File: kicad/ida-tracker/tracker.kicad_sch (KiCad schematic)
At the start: 1 part, among them J1 EURO_PWR_2x5

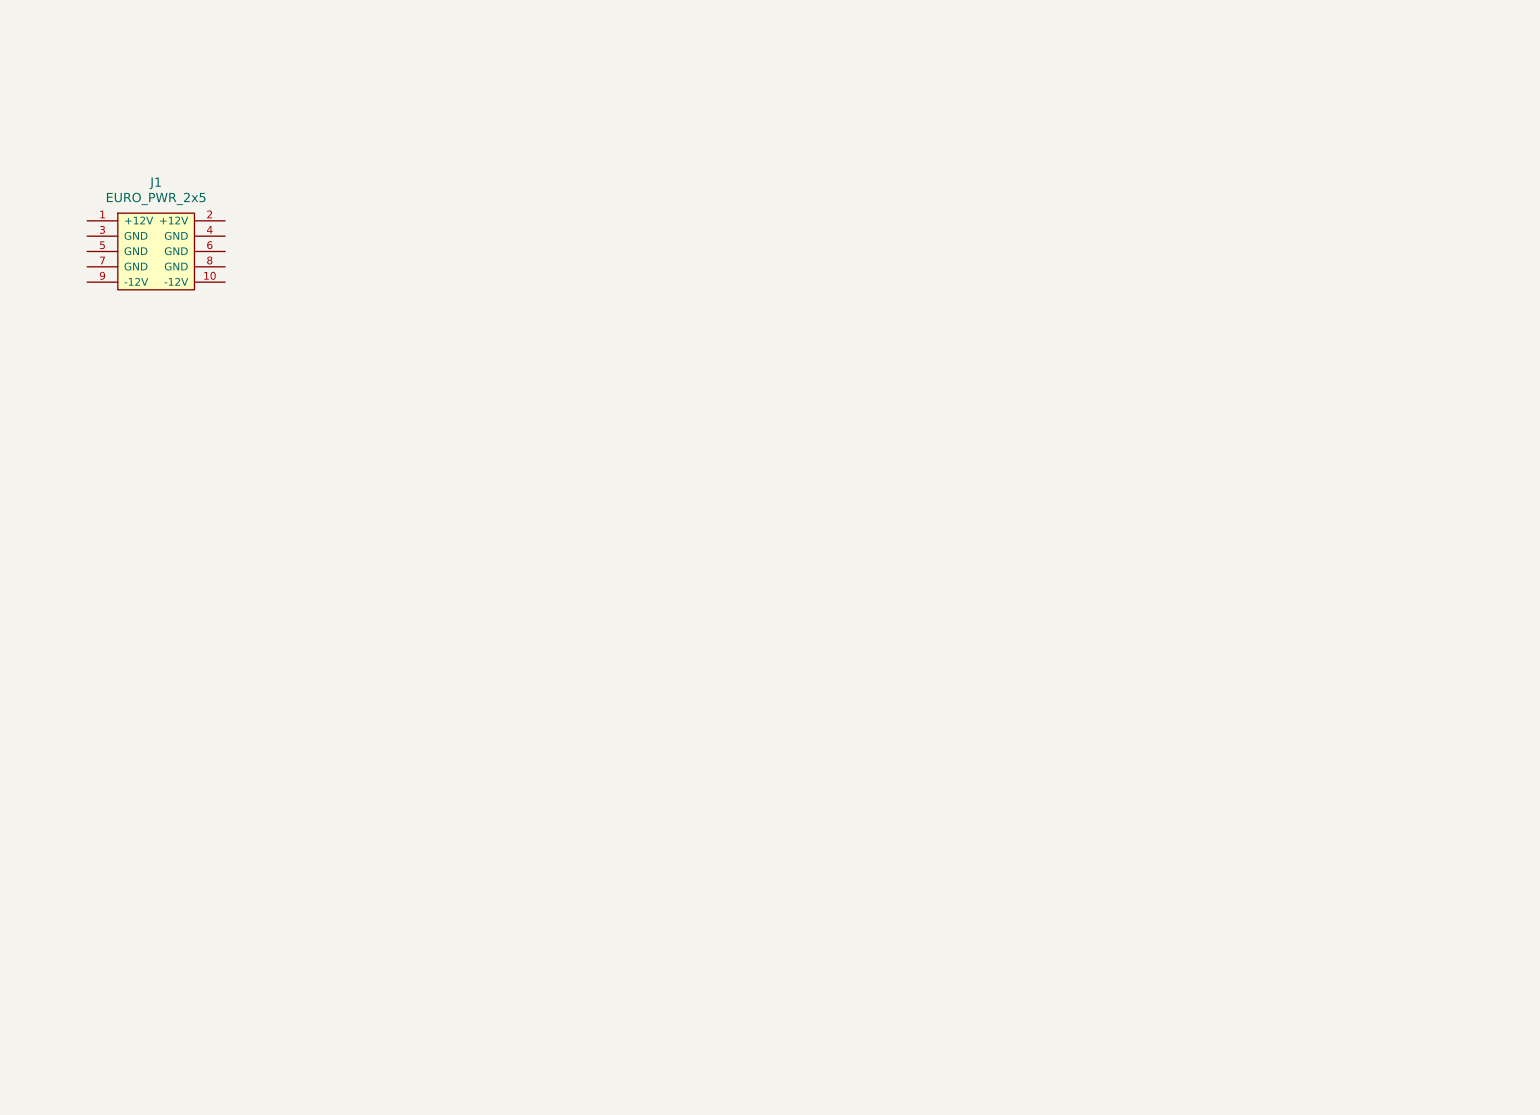
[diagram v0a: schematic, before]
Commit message: stylophone rev1
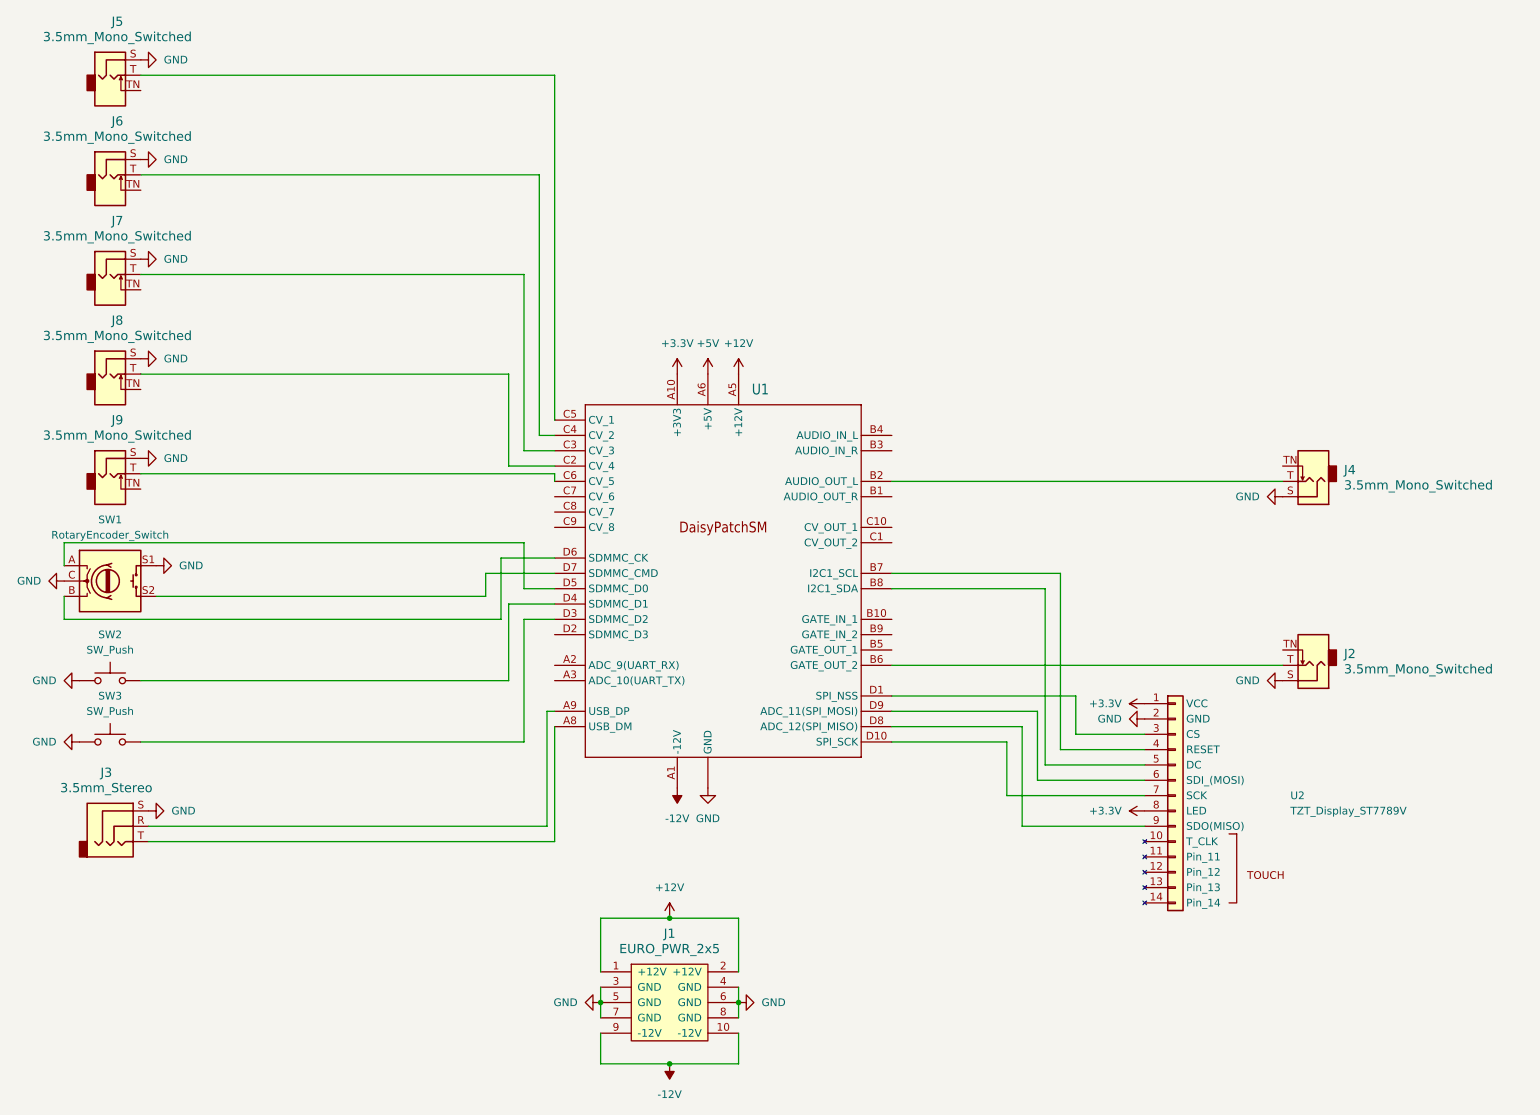
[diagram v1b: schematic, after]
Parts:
- added J2, J4, J5, J6, J7, J8, J9: 3.5mm_Mono_Switched, Connector_Audio:Jack_3.5mm_QingPu_WQP-PJ398SM_Vertical_CircularHoles, symbol KitsBlips:3.5mm_Mono_Switched
- added J3: 3.5mm_Stereo, KitsBlips:Stereo_Thonk_PJ366ST, symbol KitsBlips:3.5mm_Stereo
- added SW1: RotaryEncoder_Switch, Rotary_Encoder:RotaryEncoder_Bourns_Vertical_PEC12R-3x17F-Sxxxx, symbol Device:RotaryEncoder_Switch
- added SW2, SW3: SW_Push, Button_Switch_THT:SW_PUSH_6mm_H13mm, symbol KitsBlips:SW_Push
- added U1: ~, KitsBlips:ES_DAISY_PATCH_SM_REV1, symbol KitsBlips:Daisy_PatchSM_rev1
- added U2: TZT_Display_ST7789V, KitsBlips:TZT_Display_ST7789V, symbol KitsBlips:TZT_Display_ST7789V
- J1: footprint (none) -> KitsBlips:Pins_2x05_2.54mm_TH_Europower_shrouded
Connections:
- net +12V: now reaches J1.1 (+12V)
- net +12V: now also J1.2 (+12V), U1.A5 (+12V)
- net -12V: now reaches J1.10 (-12V)
- net -12V: now also J1.9 (-12V), U1.A1 (-12V)
- net GND: now reaches J1.3 (GND)
- net GND: now also J1.4 (GND), J1.5 (GND), J1.6 (GND), J1.7 (GND), J1.8 (GND), J2.S, J3.S, J4.S, J5.S, J6.S, J7.S, J8.S, J9.S, SW1.C, SW1.S1, SW2.1, SW3.1, U1.A4 (GND), U1.A7 (GND), U2.2 (GND)
- new net: SW2.2, U1.D4 (SDMMC_D1)
- new net: U1.D1 (SPI_NSS), U2.3 (CS)
- new net: U1.B7 (I2C1_SCL), U2.4 (RESET)
- new net: U1.B8 (I2C1_SDA), U2.5 (DC)
- new net: U1.D9 (ADC_11(SPI_MOSI)), U2.6 (SDI_(MOSI))
- new net: U1.D10 (SPI_SCK), U2.7 (SCK)
- new net: U1.D8 (ADC_12(SPI_MISO)), U2.9 (SDO(MISO))
- new net: J2.T, U1.B6 (GATE_OUT_2)
- new net: J3.T, U1.A8 (USB_DM)
- new net: J3.R, U1.A9 (USB_DP)
- new net: J4.T, U1.B2 (AUDIO_OUT_L)
- new net: J8.T, U1.C2 (CV_4)
- new net: J7.T, U1.C3 (CV_3)
- new net: J6.T, U1.C4 (CV_2)
- new net: J5.T, U1.C5 (CV_1)
- new net: J9.T, U1.C6 (CV_5)
- new net: SW3.2, U1.D3 (SDMMC_D2)
- new net: SW1.A, U1.D5 (SDMMC_D0)
- new net: SW1.B, U1.D6 (SDMMC_CK)
- new net: SW1.S2, U1.D7 (SDMMC_CMD)
- new net +3.3V: U1.A10 (+3V3), U2.1 (VCC), U2.8 (LED)
- new net +5V: U1.A6 (+5V)
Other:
- moved on the sheet: J1
